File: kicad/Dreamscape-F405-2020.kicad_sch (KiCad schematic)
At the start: 0 parts

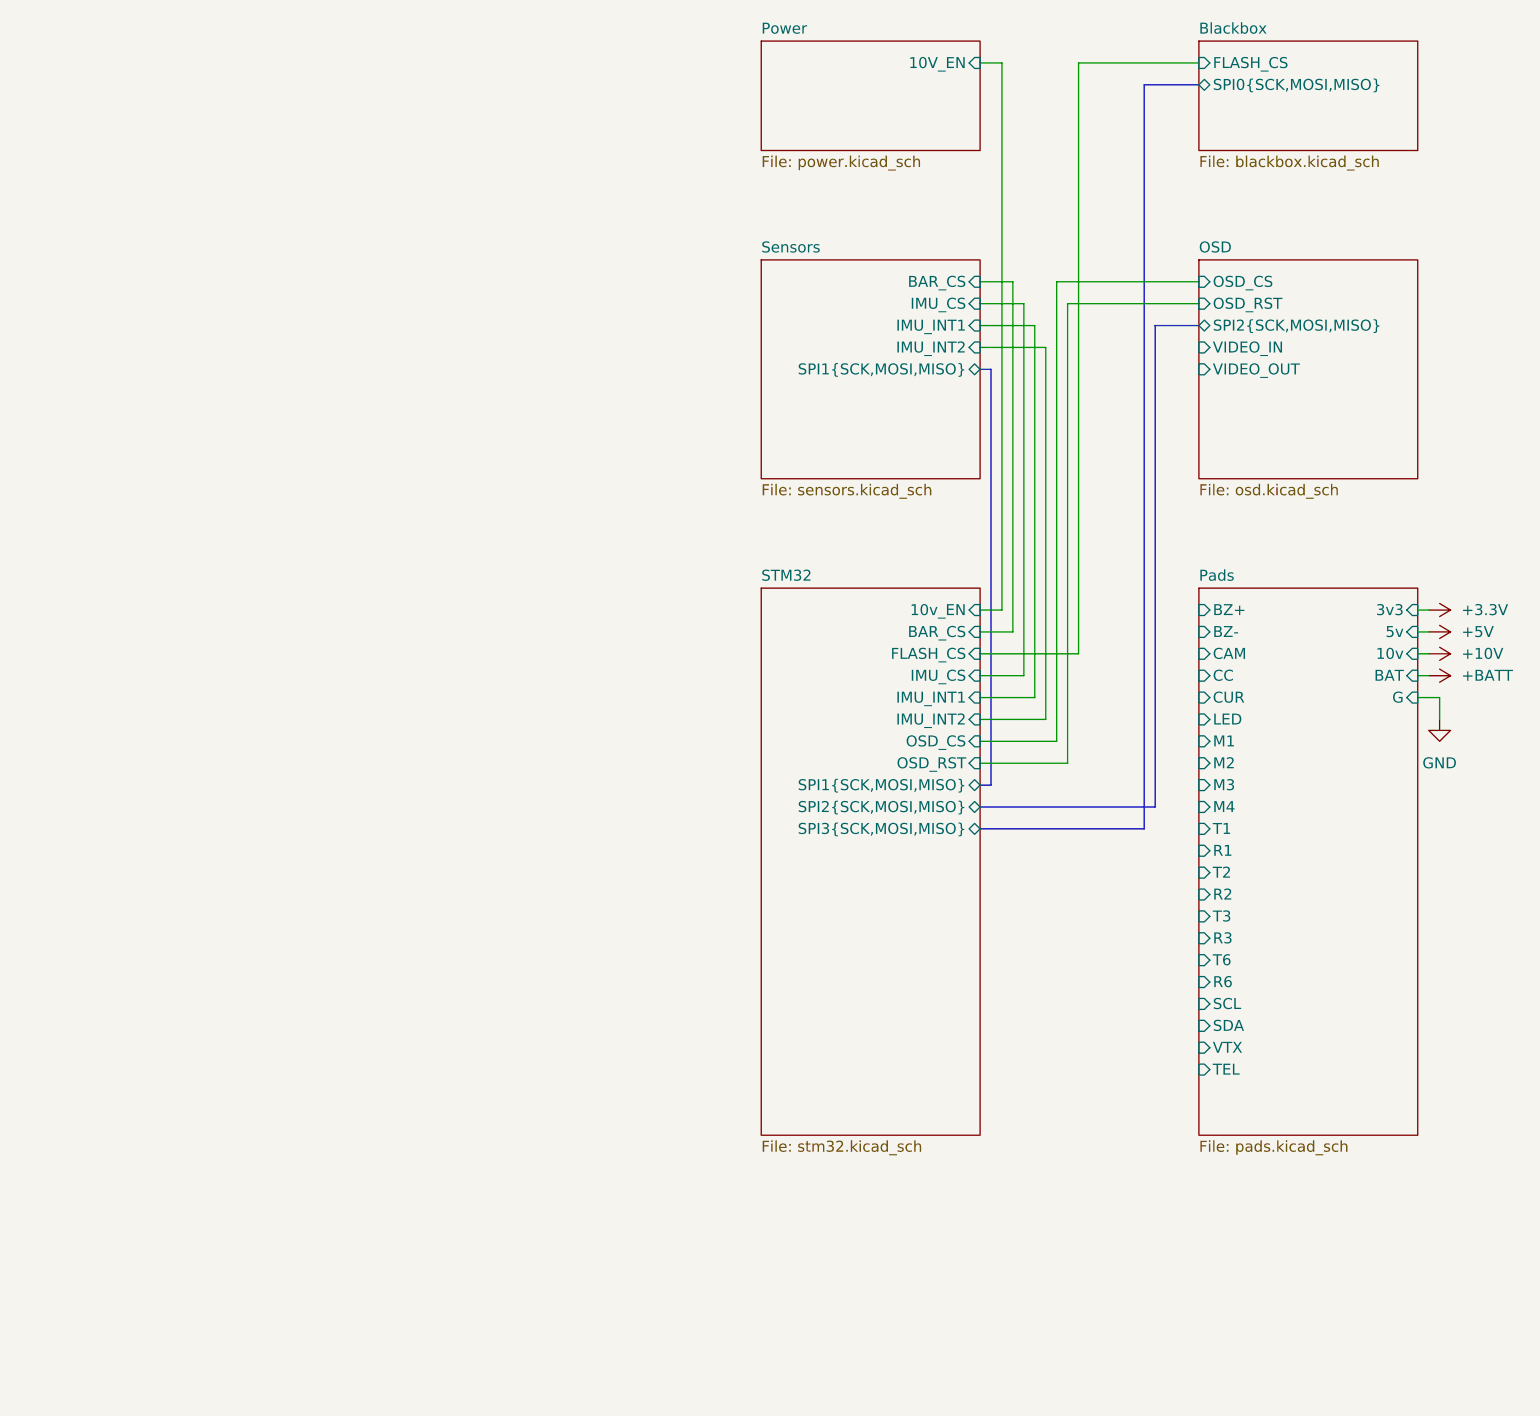
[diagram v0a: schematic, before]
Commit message: journal
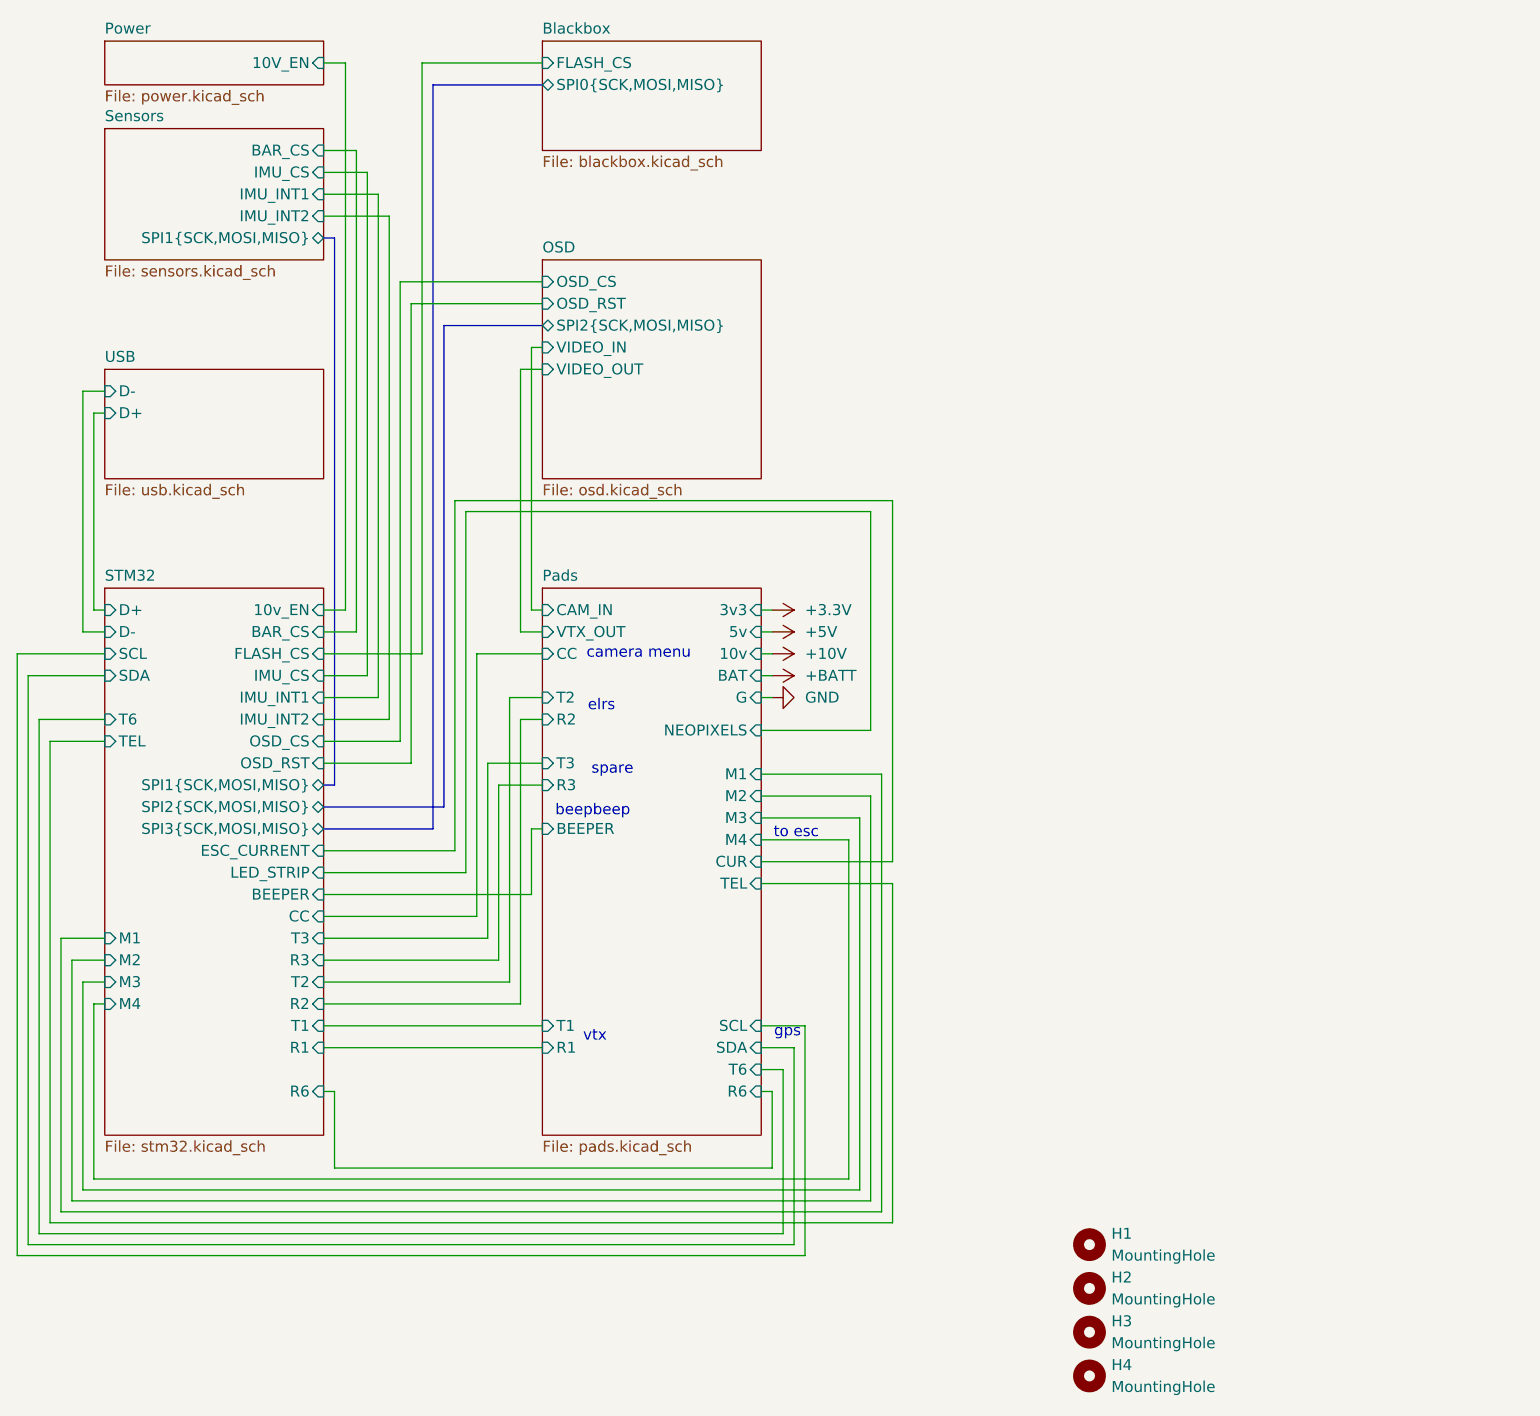
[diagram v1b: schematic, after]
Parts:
- added H1, H2, H3, H4: MountingHole, MountingHole:MountingHole_3.2mm_M3, symbol Mechanical:MountingHole
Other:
- added sheet USB (usb.kicad_sch)
- sheet Pads ports: added BEEPER, CAM_IN, NEOPIXELS, VTX_OUT; removed BZ+, BZ-, CAM, LED, VTX
- sheet STM32 ports: added BEEPER, CC, D+, D-, ESC_CURRENT, LED_STRIP, M1, M2, M3, M4, R1, R2, R3, R6, SCL, SDA, T1, T2, T3, T6, TEL; removed none
- note added: "beepbeep"
- note added: "camera menu"
- note added: "elrs"
- note added: "gps"
- note added: "spare"
- note added: "to esc"
- note added: "vtx"
